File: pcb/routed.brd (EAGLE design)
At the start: 31.8 x 31.8 mm, 85 parts, among them U2 CC430F5137IRGZR, X1 CRYSTALS-NOGND-IQXC-25, X2 FA-128

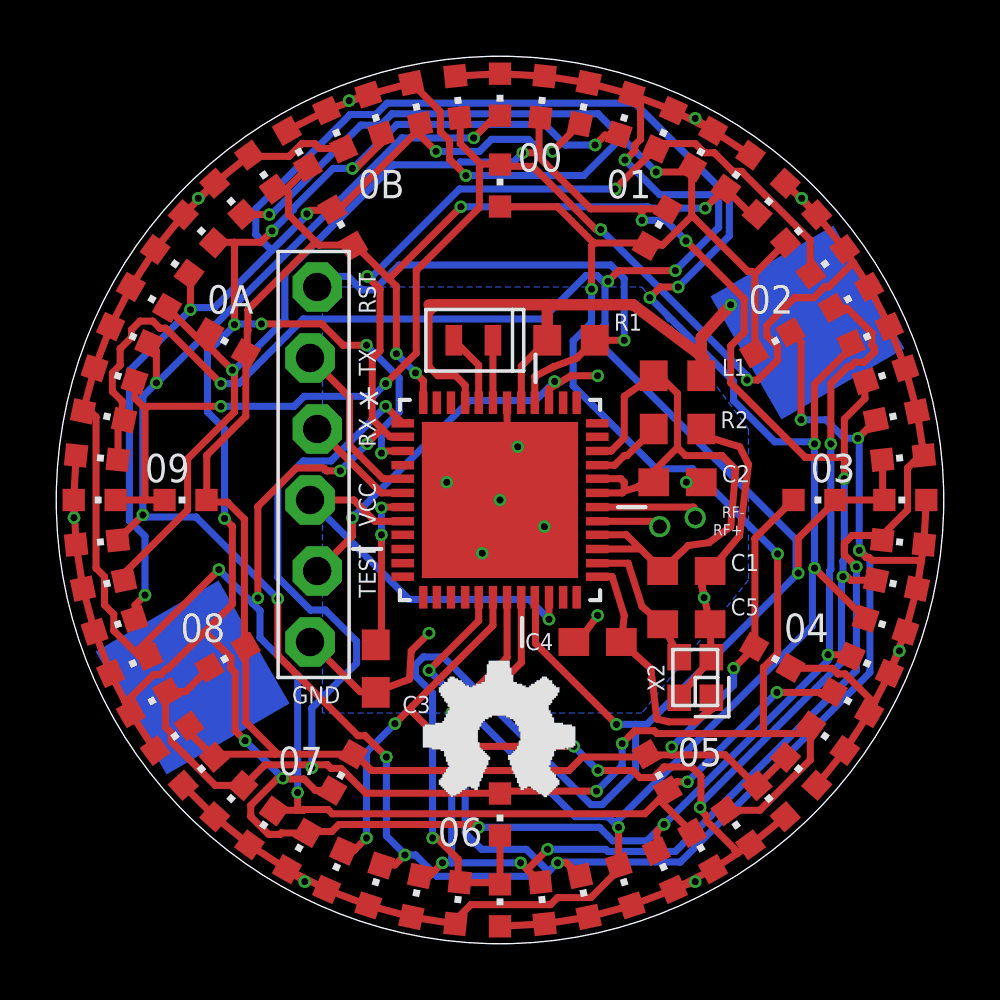
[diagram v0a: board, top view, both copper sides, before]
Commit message: as orderd v0.1
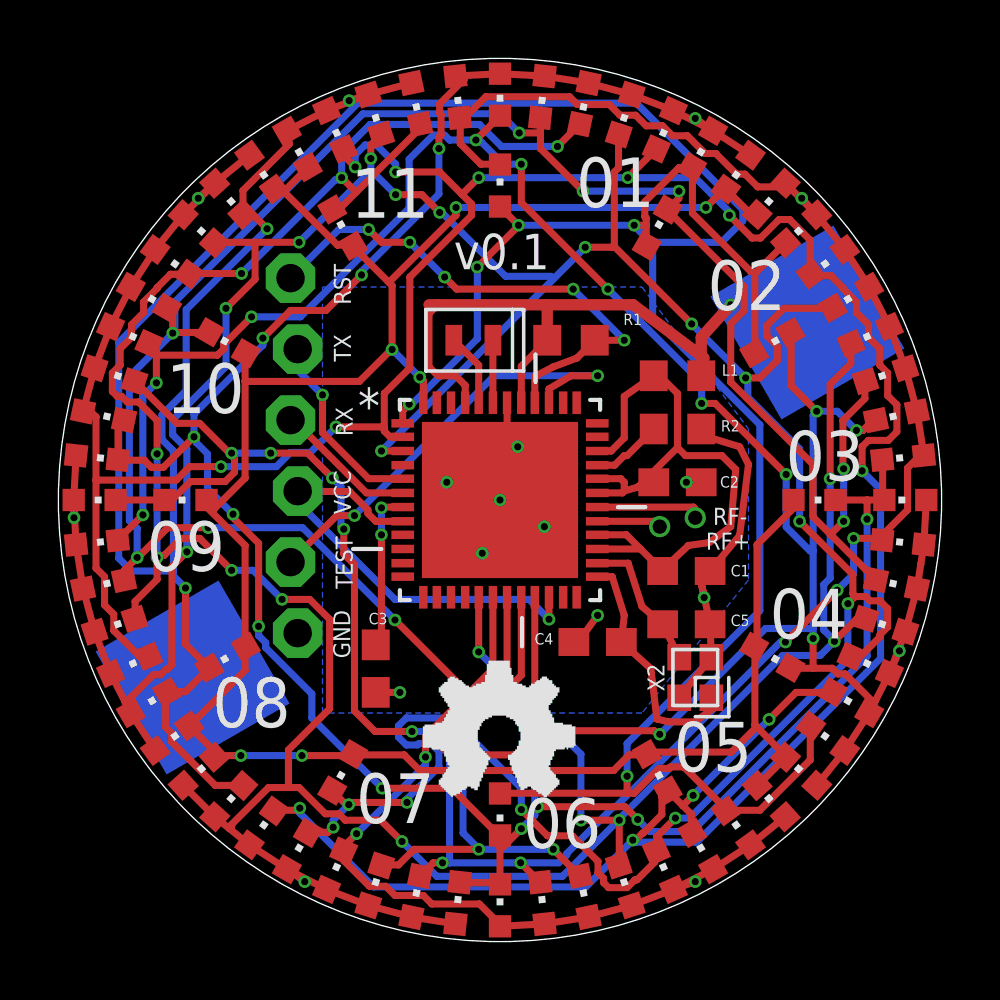
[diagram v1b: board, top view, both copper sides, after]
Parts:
- moved JP1 0.77 mm to (18.0, 27.0), flipped to the bottom
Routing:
- net B6: track 100.1 -> 121.3 mm, vias 10 -> 13
- net B0: track 107.7 -> 91.4 mm, vias 8 -> 13
- net B7: track 126.4 -> 142.2 mm, vias 10 -> 8
- net B5: track 110.3 -> 123.6 mm, vias 15 -> 18
- net B4: track 123.0 -> 116.3 mm, vias 12 -> 14
- net B1: track 98.1 -> 92.2 mm, vias 10 -> 12
- net GND: track 35.5 -> 30.1 mm
- net BSL_TEST: track 14.2 -> 16.1 mm, vias 3 -> 2
- net BSL_VCC: track 14.8 -> 16.2 mm
- net B3: track 106.0 -> 104.6 mm
- net BSL_RX: track 4.01 -> 5.10 mm
- net BSL_TX: track 6.12 -> 6.91 mm, vias 0 -> 1
- net B8: track 82.9 -> 82.2 mm
- net B2: track 109.2 -> 108.9 mm, vias 12 -> 16
- net BSL_RST: track 18.7 -> 18.9 mm, vias 1 -> 5
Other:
- board size 31.8 x 31.8 mm -> 31.6 x 31.6 mm
- board text added: "10"
- board text added: "11"
- board text added: "v0.1"
- board text removed: "00"
- board text removed: "0A"
- board text removed: "0B"
